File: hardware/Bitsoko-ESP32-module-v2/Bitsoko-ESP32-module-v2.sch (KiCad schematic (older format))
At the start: 3 parts, among them J1 CONN_02X10, J2 CONN_02X10, U1 ESP32-WROOM32-MODULE

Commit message: Changed Bitsoko ESP32 footprint to component binding in CVPCB.
Reason is detailed in commit d994a4fa
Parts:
- J1, J2: footprint narra:Pin_Header_Straight_2x10_Pitch2.54mm_staggered -> narra:Pin_Header_Straight_2x10_Pitch2.54mm_8mil_staggered
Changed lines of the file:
@@
 F 0 "J2" H 2950 3765 50  0000 C CNN
 F 1 "CONN_02X10" H 2950 3674 50  0000 C CNN
-F 2 "narra:Pin_Header_Straight_2x10_Pitch2.54mm_staggered" H 2950 1900 50  0001 C CNN
+F 2 "narra:Pin_Header_Straight_2x10_Pitch2.54mm_8mil_staggered" H 2950 1900 50  0001 C CNN
 F 3 "" H 2950 1900 50  0001 C CNN
 	1    2950 3100
@@
 F 0 "J1" H 7700 3715 50  0000 C CNN
 F 1 "CONN_02X10" H 7700 3624 50  0000 C CNN
-F 2 "narra:Pin_Header_Straight_2x10_Pitch2.54mm_staggered" H 7700 1850 50  0001 C CNN
+F 2 "narra:Pin_Header_Straight_2x10_Pitch2.54mm_8mil_staggered" H 7700 1850 50  0001 C CNN
 F 3 "" H 7700 1850 50  0001 C CNN
 	1    7700 3050

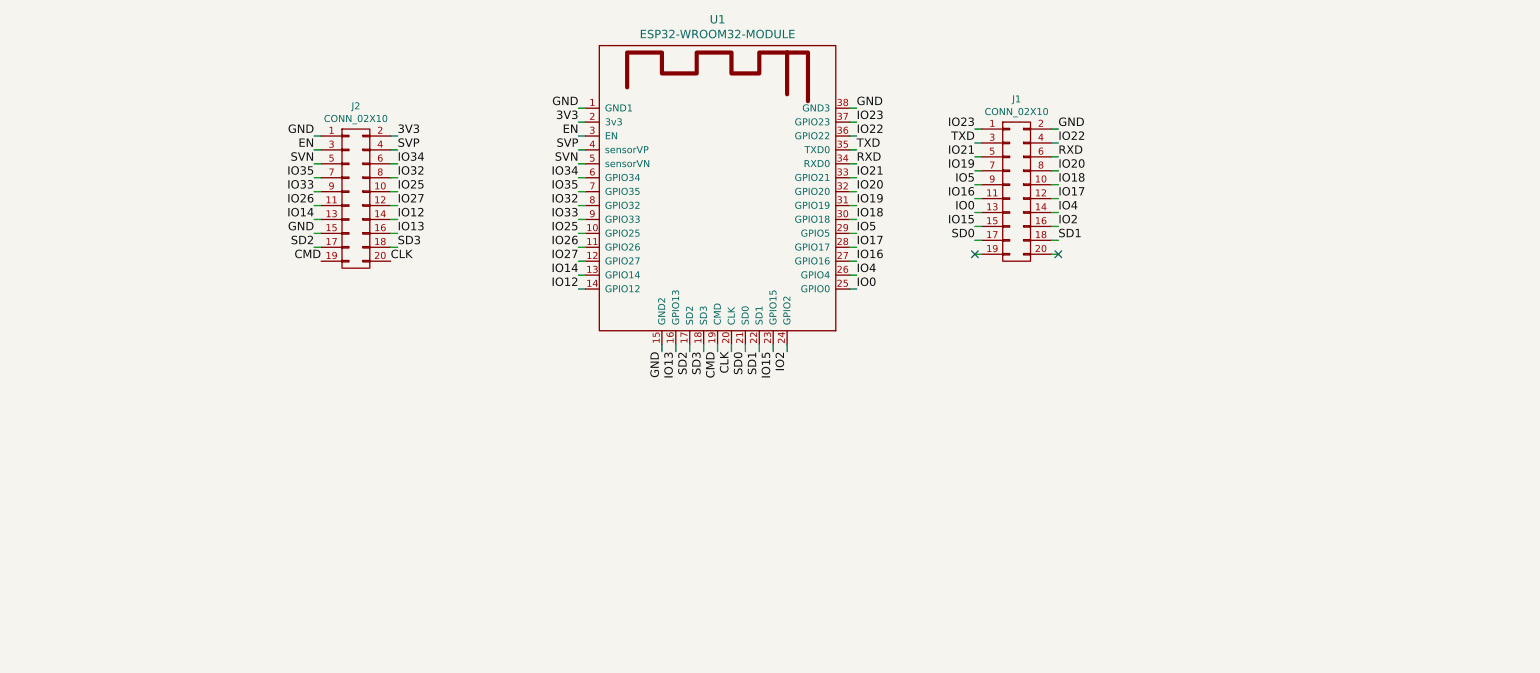
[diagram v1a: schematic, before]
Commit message: Modify ESP32 module design
1. Add 22uF 1210, 2x0.1uF 0805 decoupling capacitors.
2. Add via fence on ground under the ESP32 WROOM 32 for a solid ground connection.
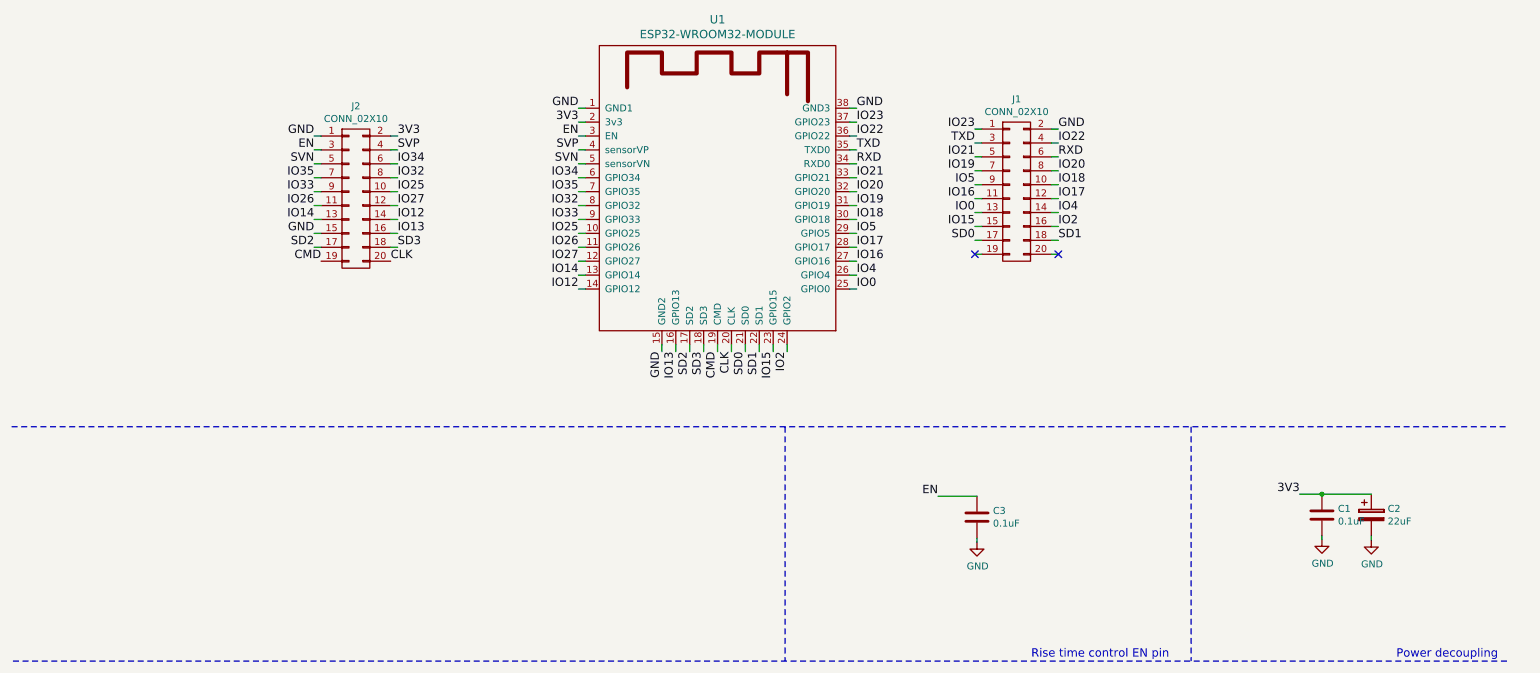
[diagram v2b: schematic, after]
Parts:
- added C1, C3: 0.1uF, Capacitors_SMD:C_0805_HandSoldering, symbol C
- added C2: 22uF, Capacitors_SMD:C_1210_HandSoldering, symbol CP
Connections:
- net 3V3: now also C1.1, C2.1
- net EN: now also C3.1
- net GND: now also C1.2, C2.2, C3.2
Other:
- note added: "Power decoupling"
- note added: "Rise time control EN pin"
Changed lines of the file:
@@
 EndData
 $EndBitmap
+Wire Notes Line
+	475  4740 11220 4740
+Wire Notes Line
+	11225 6425 470  6425
+$Comp
+L C C1
+U 1 1 59A5168F
+P 9895 5375
+F 0 "C1" H 10010 5421 50  0000 L CNN
+F 1 "0.1uF" H 10010 5330 50  0000 L CNN
+F 2 "Capacitors_SMD:C_0805_HandSoldering" H 9933 5225 50  0001 C CNN
+F 3 "" H 9895 5375 50  0001 C CNN
+	1    9895 5375
+	1    0    0    -1
+$EndComp
+$Comp
+L CP C2
+U 1 1 59A51876
+P 10250 5375
+F 0 "C2" H 10368 5421 50  0000 L CNN
+F 1 "22uF" H 10368 5330 50  0000 L CNN
+F 2 "Capacitors_SMD:C_1210_HandSoldering" H 10288 5225 50  0001 C CNN
+F 3 "" H 10250 5375 50  0001 C CNN
+	1    10250 5375
+	1    0    0    -1
+$EndComp
+Wire Wire Line
+	9735 5225 10250 5225
+$Comp
+L GND #PWR01
+U 1 1 59A51A26
+P 9895 5550
+F 0 "#PWR01" H 9895 5300 50  0001 C CNN
+F 1 "GND" H 9900 5377 50  0000 C CNN
+F 2 "" H 9895 5550 50  0001 C CNN
+F 3 "" H 9895 5550 50  0001 C CNN
+	1    9895 5550
+	1    0    0    -1
+$EndComp
+Wire Wire Line
+	9895 5550 9895 5525
+$Comp
+L GND #PWR02
+U 1 1 59A51B0B
+P 10250 5555
+F 0 "#PWR02" H 10250 5305 50  0001 C CNN
+F 1 "GND" H 10255 5382 50  0000 C CNN
+F 2 "" H 10250 5555 50  0001 C CNN
+F 3 "" H 10250 5555 50  0001 C CNN
+	1    10250 5555
+	1    0    0    -1
+$EndComp
+Text Label 9735 5225 2    60   ~ 0
+3V3
+Wire Notes Line
+	8955 4740 8955 6425
+Text Notes 10430 6410 0    60   ~ 0
+Power decoupling
+Wire Notes Line
+	6035 4740 6035 6425
+$Comp
+L C C3
+U 1 1 59A525DB
+P 7415 5390
+F 0 "C3" H 7530 5436 50  0000 L CNN
+F 1 "0.1uF" H 7530 5345 50  0000 L CNN
+F 2 "Capacitors_SMD:C_0805_HandSoldering" H 7453 5240 50  0001 C CNN
+F 3 "" H 7415 5390 50  0001 C CNN
+	1    7415 5390
+	1    0    0    -1
+$EndComp
+Wire Wire Line
+	7415 5240 7135 5240
+$Comp
+L GND #PWR03
+U 1 1 59A527F2
+P 7415 5570
+F 0 "#PWR03" H 7415 5320 50  0001 C CNN
+F 1 "GND" H 7420 5397 50  0000 C CNN
+F 2 "" H 7415 5570 50  0001 C CNN
+F 3 "" H 7415 5570 50  0001 C CNN
+	1    7415 5570
+	1    0    0    -1
+$EndComp
+Wire Wire Line
+	7415 5570 7415 5540
+Text Label 7135 5240 2    60   ~ 0
+EN
+Text Notes 7805 6410 0    60   ~ 0
+Rise time control EN pin
+Connection ~ 9895 5225
+Wire Wire Line
+	10250 5555 10250 5525
 $EndSCHEMATC
